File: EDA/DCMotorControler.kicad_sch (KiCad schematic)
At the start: 74 parts, among them J1 LOGIC Power, J10 Conn_01x04, J11 I2C1, J12 Conn_ARM_SWD_TagConnect_TC203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, J13 SPI2, J2 LOGIC Power, J3 POWER, J4 SPI1, J5 DEBUG SERIAL, J6 MOTOR, J7 LOGIC Power, J8 GPIOS, J9 Conn_01x04, Q1 PMOS, Q2 PMOS, Q3 PMOS, Q4 NMOS, Q5 PMOS, Q6 NMOS, SW1 SW_DIP_x02, U1 ICM-42670-P, U1 STM32F401CCUx, U2 AP2112K-3.3, U3 DRV8833PWP, Y1 Crystal_GND24_Small

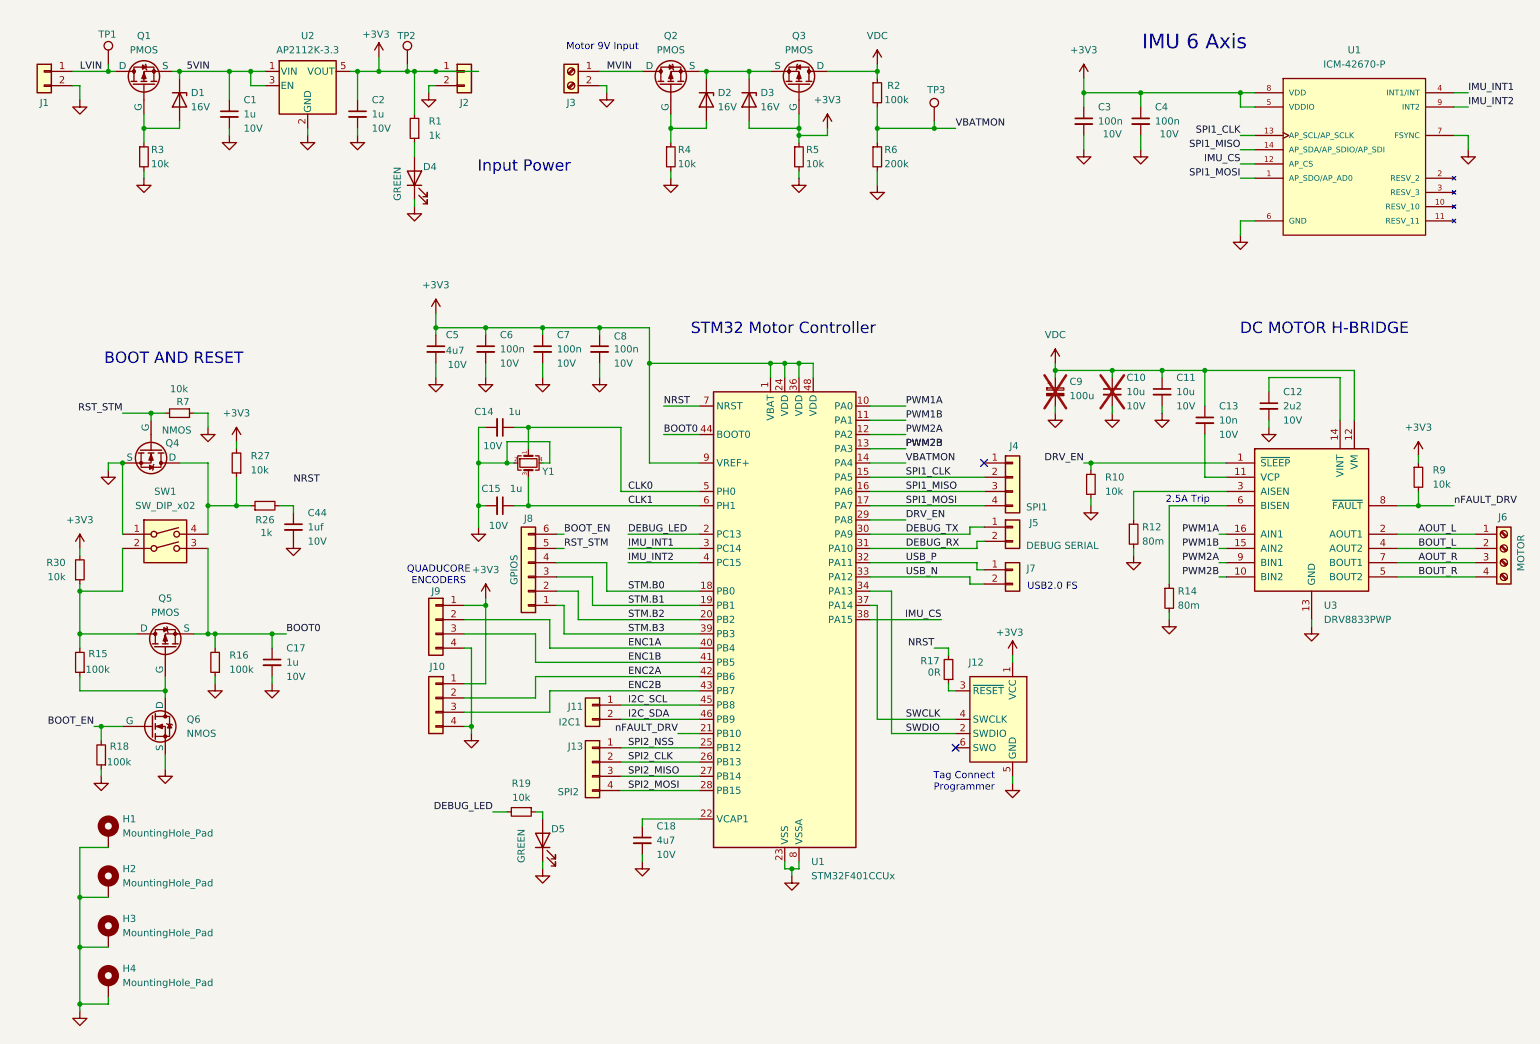
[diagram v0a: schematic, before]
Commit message: v2
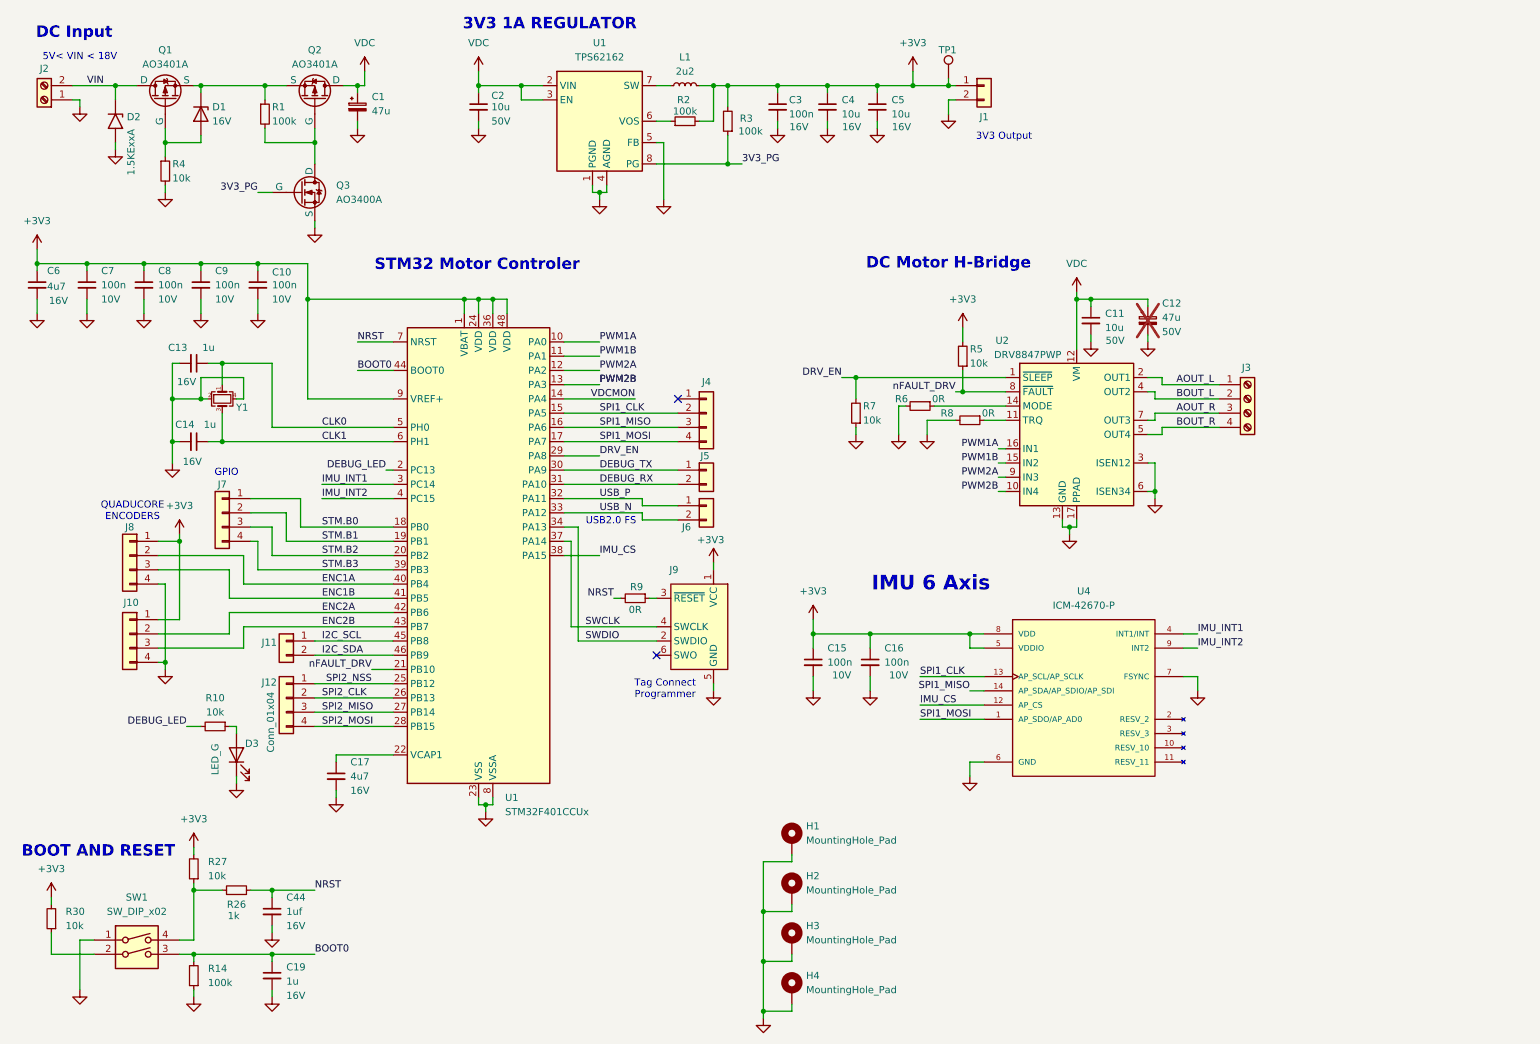
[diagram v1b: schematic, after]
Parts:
- removed C1: 1u, Capacitor_SMD:C_0402_1005Metric, symbol Device:C_Small
- removed C10: 10u, Capacitor_SMD:C_0603_1608Metric, symbol Device:C_Small
- removed C12: 2u2, Capacitor_SMD:C_0402_1005Metric, symbol Device:C_Small
- removed C13: 10n, Capacitor_SMD:C_0402_1005Metric, symbol Device:C_Small
- removed C9: 100u, Capacitor_SMD:C_0805_2012Metric, symbol Device:C_Polarized_Small
- removed D1, D3: 16V, Diode_SMD:D_0402_1005Metric, symbol Device:D_Zener
- removed D4: GREEN, Diode_SMD:D_0402_1005Metric, symbol Device:LED
- removed J1, J7: LOGIC Power, Connector_JST:JST_EH_B2B-EH-A_1x02_P2.50mm_Vertical, symbol Connector_Generic:Conn_01x02
- removed J13: SPI2, Connector_JST:JST_EH_B4B-EH-A_1x04_P2.50mm_Vertical, symbol Connector_Generic:Conn_01x04
- removed J3: POWER, TerminalBlock_Phoenix:TerminalBlock_Phoenix_MKDS-1,5-2_1x02_P5.00mm_Horizontal, symbol Connector:Screw_Terminal_01x02
- removed J6: MOTOR, TerminalBlock:TerminalBlock_Altech_AK300-4_P5.00mm, symbol Connector:Screw_Terminal_01x04
- removed J8: GPIOS, Connector_JST:JST_EH_B6B-EH-A_1x06_P2.50mm_Vertical, symbol Connector_Generic:Conn_01x06
- removed Q1, Q3, Q5: PMOS, Package_TO_SOT_SMD:TSOT-23, symbol Simulation_SPICE:PMOS
- removed Q4, Q6: NMOS, Package_TO_SOT_SMD:TSOT-23, symbol Simulation_SPICE:NMOS
- removed R1: 1k, Resistor_SMD:R_0402_1005Metric, symbol Device:R_Small
- removed R10, R9: 10k, Resistor_SMD:R_0402_1005Metric, symbol Device:R_Small
- removed R12, R14: 80m, Resistor_SMD:R_0402_1005Metric, symbol Device:R_Small
- removed R15, R18: 100k, Resistor_SMD:R_0402_1005Metric, symbol Device:R_Small
- removed TP1, TP3: TestPoint, TestPoint:TestPoint_Pad_D1.0mm, symbol Connector:TestPoint
- removed U1: ICM-42670-P, Package_LGA:LGA-14_3x2.5mm_P0.5mm_LayoutBorder3x4y, symbol Sensor_Motion:ICM-42670-P
- removed U2: AP2112K-3.3, Package_TO_SOT_SMD:SOT-23-5, symbol Regulator_Linear:AP2112K-3.3
- removed U3: DRV8833PWP, Package_SO:HTSSOP-16-1EP_4.4x5mm_P0.65mm_EP3.4x5mm_Mask2.46x2.31mm_ThermalVias, symbol Driver_Motor:DRV8833PWP
- added C1, C12: 47u, Capacitor_SMD:C_0805_2012Metric, symbol Device:C_Polarized_Small
- added C15, C16, C7: 100n, Capacitor_SMD:C_0402_1005Metric, symbol Device:C_Small
- added C5: 10u, Capacitor_SMD:C_0603_1608Metric, symbol Device:C_Small
- added D2: 1.5KExxA, Diode_SMD:D_0805_2012Metric, symbol Diode:1.5KExxA
- added J12, J7: Conn_01x04, Connector_JST:JST_XH_B4B-XH-A_1x04_P2.50mm_Vertical, symbol Connector_Generic:Conn_01x04
- added J2: Conn_01x02, TerminalBlock_Phoenix:TerminalBlock_Phoenix_MKDS-1,5-2_1x02_P5.00mm_Horizontal, symbol Connector:Screw_Terminal_01x02
- added J3: Conn_01x04, TerminalBlock:TerminalBlock_Altech_AK300-4_P5.00mm, symbol Connector:Screw_Terminal_01x04
- added J6: Conn_01x02, Connector_JST:JST_XH_B2B-XH-A_1x02_P2.50mm_Vertical, symbol Connector_Generic:Conn_01x02
- added L1: 2u2, Inductor_SMD:L_0603_1608Metric, symbol Device:L_Small
- added Q2: AO3401A, Package_TO_SOT_SMD:TSOT-23, symbol Simulation_SPICE:PMOS
- added Q3: AO3400A, Package_TO_SOT_SMD:TSOT-23, symbol Simulation_SPICE:NMOS
- added R5: 10k, Resistor_SMD:R_0402_1005Metric, symbol Device:R_Small
- added R8: 0R, Resistor_SMD:R_0402_1005Metric, symbol Device:R_Small
- added U1: TPS62162, Package_SO:MSOP-8_3x3mm_P0.65mm, symbol Regulator_Switching:TPS62162
- added U2: DRV8847PWP, Package_SO:HTSSOP-16-1EP_4.4x5mm_P0.65mm_EP3.4x5mm_Mask2.46x2.31mm_ThermalVias, symbol Driver_Motor:DRV8847PWP
- added U4: ICM-42670-P, Package_LGA:LGA-14_3x2.5mm_P0.5mm_LayoutBorder3x4y, symbol Sensor_Motion:ICM-42670-P
- C11: Voltage 10V -> 50V
- C13: renamed from C14; Voltage 10V -> 16V
- C14: renamed from C15; Voltage 10V -> 16V
- C17: renamed from C18; Voltage 10V -> 16V
- C19: renamed from C17; Voltage 10V -> 16V
- C2: value 1u -> 10u; footprint Capacitor_SMD:C_0402_1005Metric -> Capacitor_SMD:C_0603_1608Metric; Voltage 10V -> 50V
- C3, C44: Voltage 10V -> 16V
- C4: value 100n -> 10u; footprint Capacitor_SMD:C_0402_1005Metric -> Capacitor_SMD:C_0603_1608Metric; Voltage 10V -> 16V
- C6: renamed from C5; Voltage 10V -> 16V
- D3: renamed from D5; value GREEN -> LED_G
- J1: renamed from J2; value LOGIC Power -> Conn_01x02; footprint Connector_JST:JST_EH_B2B-EH-A_1x02_P2.50mm_Vertical -> TerminalBlock_Phoenix:TerminalBlock_Phoenix_MKDS-1,5-2_1x02_P5.00mm_Horizontal
- J10: footprint Connector_JST:JST_EH_B4B-EH-A_1x04_P2.50mm_Vertical -> Connector_JST:JST_XH_B4B-XH-A_1x04_P2.50mm_Vertical
- J11: value I2C1 -> Conn_01x02; footprint Connector_JST:JST_EH_B2B-EH-A_1x02_P2.50mm_Vertical -> Connector_JST:JST_XH_B2B-XH-A_1x02_P2.50mm_Vertical
- J4: value SPI1 -> Conn_01x04; footprint Connector_JST:JST_EH_B4B-EH-A_1x04_P2.50mm_Vertical -> Connector_JST:JST_XH_B4B-XH-A_1x04_P2.50mm_Vertical
- J5: value DEBUG SERIAL -> Conn_01x02; footprint Connector_JST:JST_EH_B2B-EH-A_1x02_P2.50mm_Vertical -> Connector_JST:JST_XH_B2B-XH-A_1x02_P2.50mm_Vertical
- J8: renamed from J9; footprint Connector_JST:JST_EH_B4B-EH-A_1x04_P2.50mm_Vertical -> Connector_JST:JST_XH_B4B-XH-A_1x04_P2.50mm_Vertical
- Q1: renamed from Q2; value PMOS -> AO3401A; JLC_PN (none) -> C15127; MFN (none) -> Alpha & Omega Semicon; MPN (none) -> AO3401A
- R1: renamed from R5; value 10k -> 100k; Tollerance (none) -> 1%
- R10: renamed from R19; Tollerance (none) -> 1%
- R14: renamed from R16; Tollerance (none) -> 1%
- R2, R27, R30, R4, R7: Tollerance (none) -> 1%
- R3: value 10k -> 100k; Tollerance (none) -> 1%
- R6: value 200k -> 0R; Tollerance (none) -> 1%
- R9: renamed from R17; Tollerance (none) -> 1%
- U1: MFN (none) -> STM32F401CCU6E
- renumbered C8 to C10, C6 to C8, C7 to C9, D2 to D1, J12 to J9, TP2 to TP1
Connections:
- net RST_STM is gone; now on net DRV_EN: R7.2
- net +3V3: now also R2.2, R3.2, C15.1, C16.1, C5.1, C7.1, L1.2, R5.2, U4.5 (VDDIO), U4.8 (VDD); no longer C2.1, R1.1
- net AOUT_L: now also J3.1 (Pin_1), U2.2 (OUT1)
- net AOUT_R: now also J3.3 (Pin_3), U2.7 (OUT3)
- net BOUT_L: now also J3.2 (Pin_2), U2.4 (OUT2)
- net BOUT_R: now also J3.4 (Pin_4), U2.5 (OUT4)
- net DRV_EN: now also U2.1 (~{SLEEP})
- net GND: now also C1.2, C12.2, C15.2, C16.2, C5.2, C7.2, D2.2 (A2), J2.1 (Pin_1), Q3.3 (S), R8.2, U1.1 (PGND), U1.4 (AGND), U1.5 (FB), U2.13 (GND), U2.17 (PPAD), U2.3 (ISEN12), U2.6 (ISEN34), U4.6 (GND), U4.7 (FSYNC); no longer R1.2, R3.2
- net IMU_CS: now also U4.12 (AP_CS)
- net IMU_INT1: now also U4.4 (INT1/INT)
- net IMU_INT2: now also U4.9 (INT2)
- net NRST: now also C44.1, R26.2
- net PWM1A: now also U2.16 (IN1)
- net PWM1B: now also U2.15 (IN2)
- net PWM2A: now also U2.9 (IN3)
- net PWM2B: now also U2.10 (IN4)
- net SPI1_CLK: now also U4.13 (AP_SCL/AP_SCLK)
- net SPI1_MISO: now also U4.14 (AP_SDA/AP_SDIO/AP_SDI)
- net SPI1_MOSI: now also U4.1 (AP_SDO/AP_AD0)
- net SPI2_CLK: now also J12.2 (Pin_2)
- net SPI2_MISO: now also J12.3 (Pin_3)
- net SPI2_MOSI: now also J12.4 (Pin_4)
- net SPI2_NSS: now also J12.1 (Pin_1)
- net STM.B0: now also J7.1 (Pin_1)
- net STM.B1: now also J7.2 (Pin_2)
- net STM.B2: now also J7.3 (Pin_3)
- net STM.B3: now also J7.4 (Pin_4)
- net USB_N: now also J6.2 (Pin_2)
- net USB_P: now also J6.1 (Pin_1)
- net VDC: now also C2.1, C1.1, C12.1, Q2.1 (D), U1.2 (VIN), U1.3 (EN), U2.12 (VM); no longer R2.1
- net nFAULT_DRV: now also R5.1, U2.8 (~{FAULT})
- net at D1.1 (K), Q1.3 (S): now also R1.1, Q2.3 (S)
- net 3V3_PG: now reaches R3.1
- net 3V3_PG: now also Q3.2 (G), U1.8 (PG)
- net MVIN renamed VIN
- net VIN: now also D2.1 (A1), J2.2 (Pin_2)
- removed net VBATMON: R2.2, R6.1, U1.14 (PA4)
- new net: R2.1, U1.6 (VOS)
- new net: L1.1, U1.7 (SW)
- new net: Q2.2 (G), Q3.1 (D), R1.2
- new net: R8.1, U2.11 (TRQ)
- new net: R6.1, U2.14 (MODE)
- new net VDCMON: U1.14 (PA4)
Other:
- note added: "3V3 1A REGULATOR"
- note added: "3V3 Output"
- note added: "5V< VIN < 18V"
- note added: "DC Input"
- note added: "DC Motor H-Bridge"
- note added: "GPIO"
- note added: "STM32 Motor Controler"
- note removed: "2.5A Trip"
- note removed: "DC MOTOR H-BRIDGE"
- note removed: "Input Power"
- note removed: "Motor 9V Input"
- note removed: "STM32 Motor Controller"
- moved on the sheet: C10, C13, C14, C17, C19, C44, C6, C8, C9, D1, D3, H1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
